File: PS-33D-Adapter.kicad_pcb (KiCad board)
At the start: 2 copper layers, 8 parts, among them J1 CONN_05, J2 Conn_02x04_Counter_Clockwise, Q1 MOSFET-NCH-BSS138, Q2 MOSFET-NCH-BSS138

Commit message: feat: update mask clearance, mask min width
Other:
- rule pad_to_mask_clearance: 0 -> 0.0508

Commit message: feat: update setup
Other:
- net class Default: clearance 0.2 -> 0.254; trace_width 0.25 -> 0.254; via_dia 0.8 -> 0.762; via_drill 0.4 -> 0.381
- rule trace_clearance: 0.2 -> 0.254
- rule trace_min: 0.2 -> 0.1524
- rule via_min_drill: 0.3 -> 0.254
- rule via_min_size: 0.4 -> 0.508

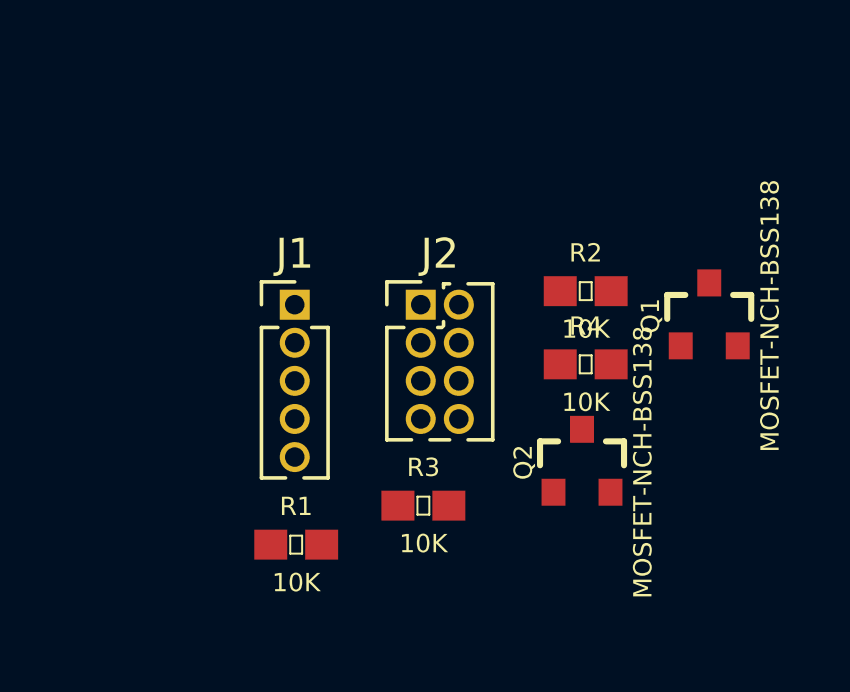
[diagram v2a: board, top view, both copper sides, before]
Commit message: feat: update pcb
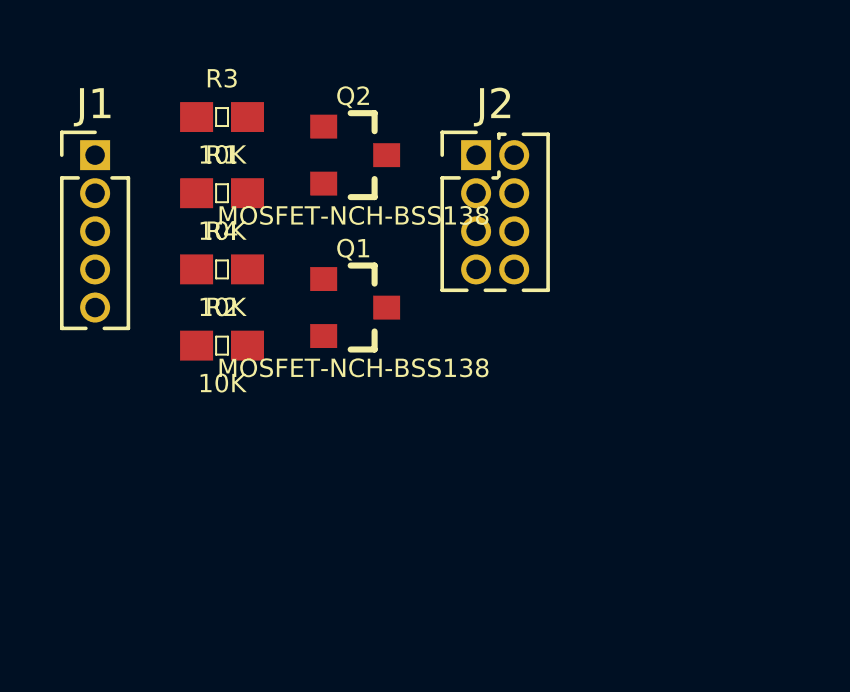
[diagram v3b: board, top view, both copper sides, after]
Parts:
- moved R3 14.6 mm to (151.6, 77.5)
- moved Q2 12.8 mm to (155.9, 78.7), turned to 270 degrees
- moved R4 12.5 mm to (151.6, 82.5)
- moved R2 12.3 mm to (151.6, 85.1)
- moved R1 12.0 mm to (151.6, 80.0)
- moved Q1 11.9 mm to (155.9, 83.8), turned to 270 degrees
- moved J1 8.32 mm to (147.3, 78.7)
- moved J2 5.32 mm to (160.0, 78.7)
